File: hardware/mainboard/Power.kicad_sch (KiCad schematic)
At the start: 48 parts, among them IC1 3.3V/0.5A, IC2 TPS54202HDDCR, Q4 SI2347DS-T1-GE3, U4 TPS2113PWR

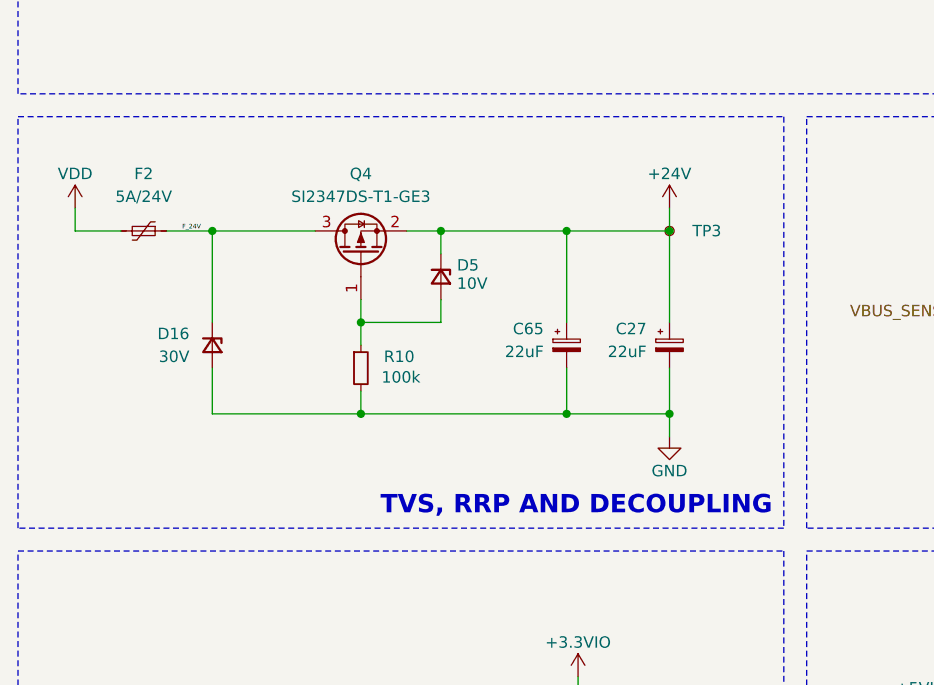
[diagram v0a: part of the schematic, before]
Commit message: chore: sync
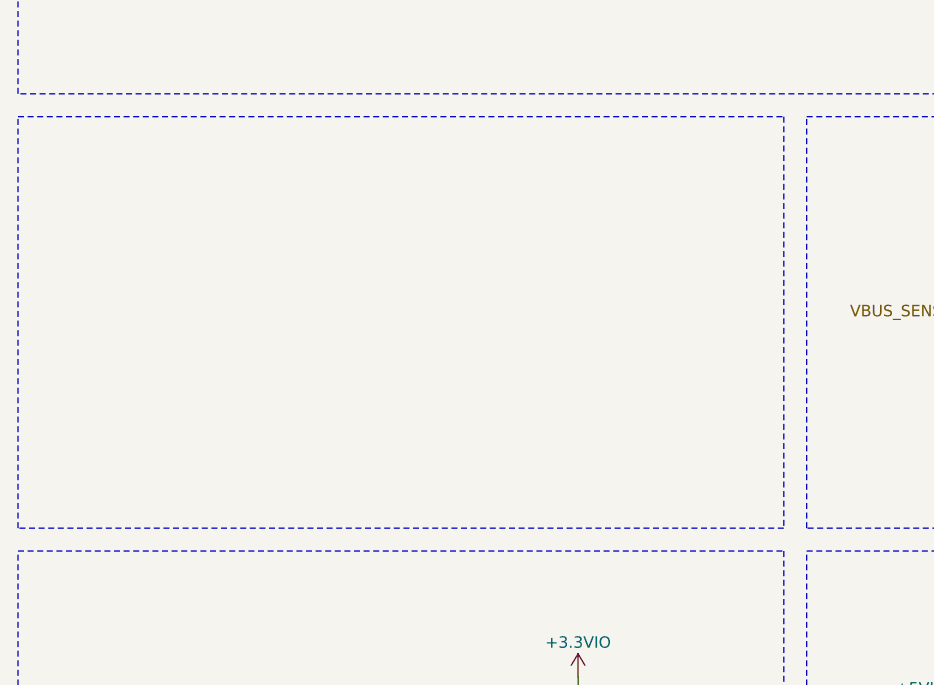
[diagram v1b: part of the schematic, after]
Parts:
- removed C27, C65: 22uF, Capacitor_SMD:CP_Elec_4x5.8, symbol Device:C_Polarized_Small
- removed D16: 30V, Diode_SMD:D_SOD-123, symbol Device:D_Zener_Small
- removed D5: 10V, Diode_SMD:D_SOD-123, symbol Device:D_Zener_Small
- removed F2: 5A/24V, Fuse:Fuse_2920_7451Metric, symbol Device:Polyfuse_Small
- removed Q4: SI2347DS-T1-GE3, Package_TO_SOT_SMD:SOT-23-3, symbol Transistor_FET:Q_PMOS_GSD
- removed R10: 100k, Resistor_SMD:R_0603_1608Metric_Pad0.98x0.95mm_HandSolder, symbol Device:R_Small
- removed TP3: TestPoint_Small, TestPoint:TestPoint_THTPad_D1.0mm_Drill0.5mm, symbol Connector:TestPoint_Small
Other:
- note removed: "TVS, RRP AND DECOUPLING"
